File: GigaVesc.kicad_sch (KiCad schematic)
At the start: 0 parts

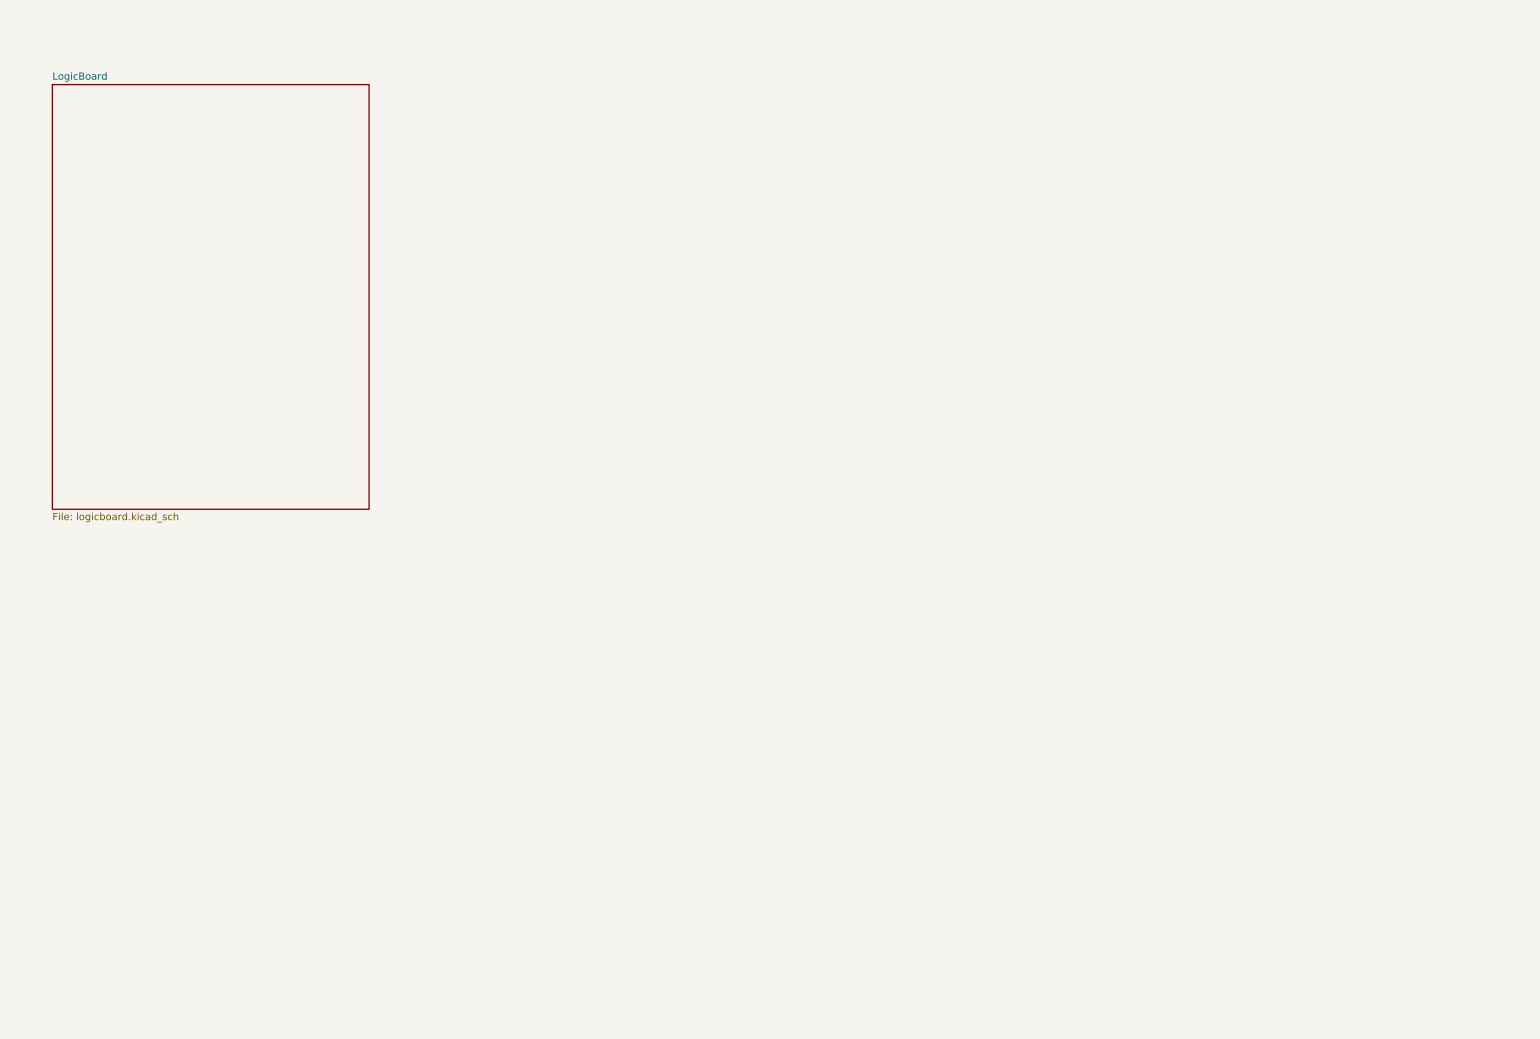
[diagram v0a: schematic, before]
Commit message: initial
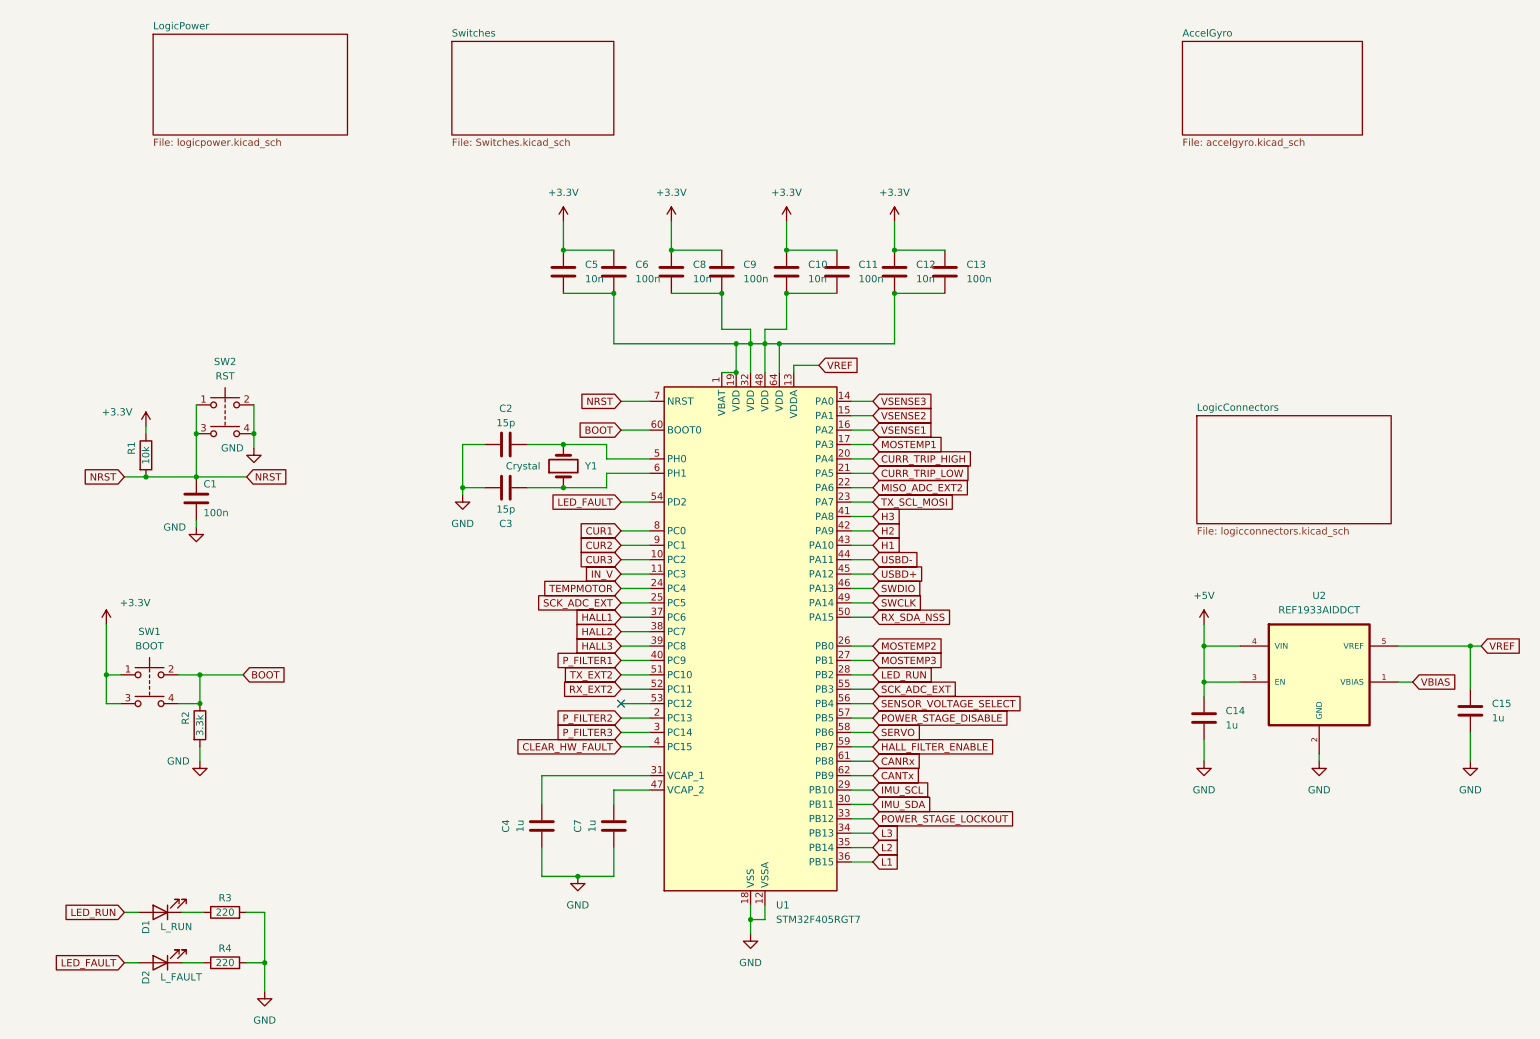
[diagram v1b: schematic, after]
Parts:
- added C1, C11, C13, C6, C9: 100n, Capacitor_SMD:C_0805_2012Metric, symbol Device:C
- added C10, C12, C5, C8: 10n, Capacitor_SMD:C_0805_2012Metric, symbol Device:C
- added C14, C15, C4, C7: 1u, Capacitor_SMD:C_0805_2012Metric, symbol Device:C
- added C2, C3: 15p, Capacitor_SMD:C_0805_2012Metric, symbol Device:C
- added D1: L_RUN, LED_SMD:LED_0805_2012Metric, symbol Device:LED
- added D2: L_FAULT, LED_SMD:LED_0805_2012Metric, symbol Device:LED
- added R1: 10k, Resistor_SMD:R_0805_2012Metric, symbol Device:R
- added R2: 3.3k, Resistor_SMD:R_0805_2012Metric, symbol Device:R
- added R3, R4: 220, Resistor_SMD:R_0805_2012Metric, symbol Device:R
- added SW1: BOOT, Button_Switch_SMD:SW_SPST_CK_RS282G05A3, symbol Switch:SW_Push_Dual
- added SW2: RST, Button_Switch_SMD:SW_SPST_CK_RS282G05A3, symbol Switch:SW_Push_Dual
- added U1: STM32F405RGT7, Package_QFP:LQFP-64_10x10mm_P0.5mm, symbol MCU_ST_STM32F4:STM32F405RGTx
- added U2: REF1933AIDDCT, Package_TO_SOT_SMD:SOT-23-5, symbol GigaVescSymbols:REF1933AIDDCT
- added Y1: Crystal, Crystal:Crystal_SMD_HC49-SD, symbol Device:Crystal
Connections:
- new net: C10.2, C11.2, C12.2, C13.2, C5.2, C6.2, C8.2, C9.2, U1.1 (VBAT), U1.19 (VDD), U1.32 (VDD), U1.48 (VDD), U1.64 (VDD)
- new net: D2.1 (K), R4.1
- new net: C2.1, U1.5 (PH0), Y1.2
- new net: D1.1 (K), R3.1
- new net: C4.1, U1.31 (VCAP_1)
- new net: C7.1, U1.47 (VCAP_2)
- new net: C3.2, U1.6 (PH1), Y1.1
- new net +3.3V: C10.1, C11.1, C12.1, C13.1, C5.1, C6.1, C8.1, C9.1, R1.1, SW1.1, SW1.3
- new net +5V: C14.1, U2.3 (EN), U2.4 (VIN)
- new net BOOT: R2.1, SW1.2, SW1.4, U1.60 (BOOT0)
- new net CANRx: U1.61 (PB8)
- new net CANTx: U1.62 (PB9)
- new net CLEAR_HW_FAULT: U1.4 (PC15)
- new net CUR1: U1.8 (PC0)
- new net CUR2: U1.9 (PC1)
- new net CUR3: U1.10 (PC2)
- new net CURR_TRIP_HIGH: U1.20 (PA4)
- new net CURR_TRIP_LOW: U1.21 (PA5)
- new net GND: C1.2, C14.2, C15.2, C2.2, C3.1, C4.2, C7.2, R2.2, R3.2, R4.2, SW2.2, SW2.4, U1.12 (VSSA), U1.18 (VSS), U1.63 (VSS), U2.2 (GND)
- new net H1: U1.43 (PA10)
- new net H2: U1.42 (PA9)
- new net H3: U1.41 (PA8)
- new net HALL1: U1.37 (PC6)
- new net HALL2: U1.38 (PC7)
- new net HALL3: U1.39 (PC8)
- new net HALL_FILTER_ENABLE: U1.59 (PB7)
- new net IMU_SCL: U1.29 (PB10)
- new net IMU_SDA: U1.30 (PB11)
- new net IN_V: U1.11 (PC3)
- new net L1: U1.36 (PB15)
- new net L2: U1.35 (PB14)
- new net L3: U1.34 (PB13)
- new net LED_FAULT: D2.2 (A), U1.54 (PD2)
- new net LED_RUN: D1.2 (A), U1.28 (PB2)
- new net MISO_ADC_EXT2: U1.22 (PA6)
- new net MOSTEMP1: U1.17 (PA3)
- new net MOSTEMP2: U1.26 (PB0)
- new net MOSTEMP3: U1.27 (PB1)
- new net NRST: C1.1, R1.2, SW2.1, SW2.3, U1.7 (NRST)
- new net POWER_STAGE_DISABLE: U1.57 (PB5)
- new net POWER_STAGE_LOCKOUT: U1.33 (PB12)
- new net P_FILTER1: U1.40 (PC9)
- new net P_FILTER2: U1.2 (PC13)
- new net P_FILTER3: U1.3 (PC14)
- new net RX_EXT2: U1.52 (PC11)
- new net RX_SDA_NSS: U1.50 (PA15)
- new net SCK_ADC_EXT: U1.25 (PC5), U1.55 (PB3)
- new net SENSOR_VOLTAGE_SELECT: U1.56 (PB4)
- new net SERVO: U1.58 (PB6)
- new net SWCLK: U1.49 (PA14)
- new net SWDIO: U1.46 (PA13)
- new net TEMPMOTOR: U1.24 (PC4)
- new net TX_EXT2: U1.51 (PC10)
- new net TX_SCL_MOSI: U1.23 (PA7)
- new net USBD+: U1.45 (PA12)
- new net USBD-: U1.44 (PA11)
- new net VBIAS: U2.1 (VBIAS)
- new net VREF: C15.1, U1.13 (VDDA), U2.5 (VREF)
- new net VSENSE1: U1.16 (PA2)
- new net VSENSE2: U1.15 (PA1)
- new net VSENSE3: U1.14 (PA0)
- no-connect marks 0 -> 1
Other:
- removed sheet LogicBoard
- added sheet AccelGyro (accelgyro.kicad_sch)
- added sheet LogicConnectors (logicconnectors.kicad_sch)
- added sheet LogicPower (logicpower.kicad_sch)
- added sheet Switches (Switches.kicad_sch)

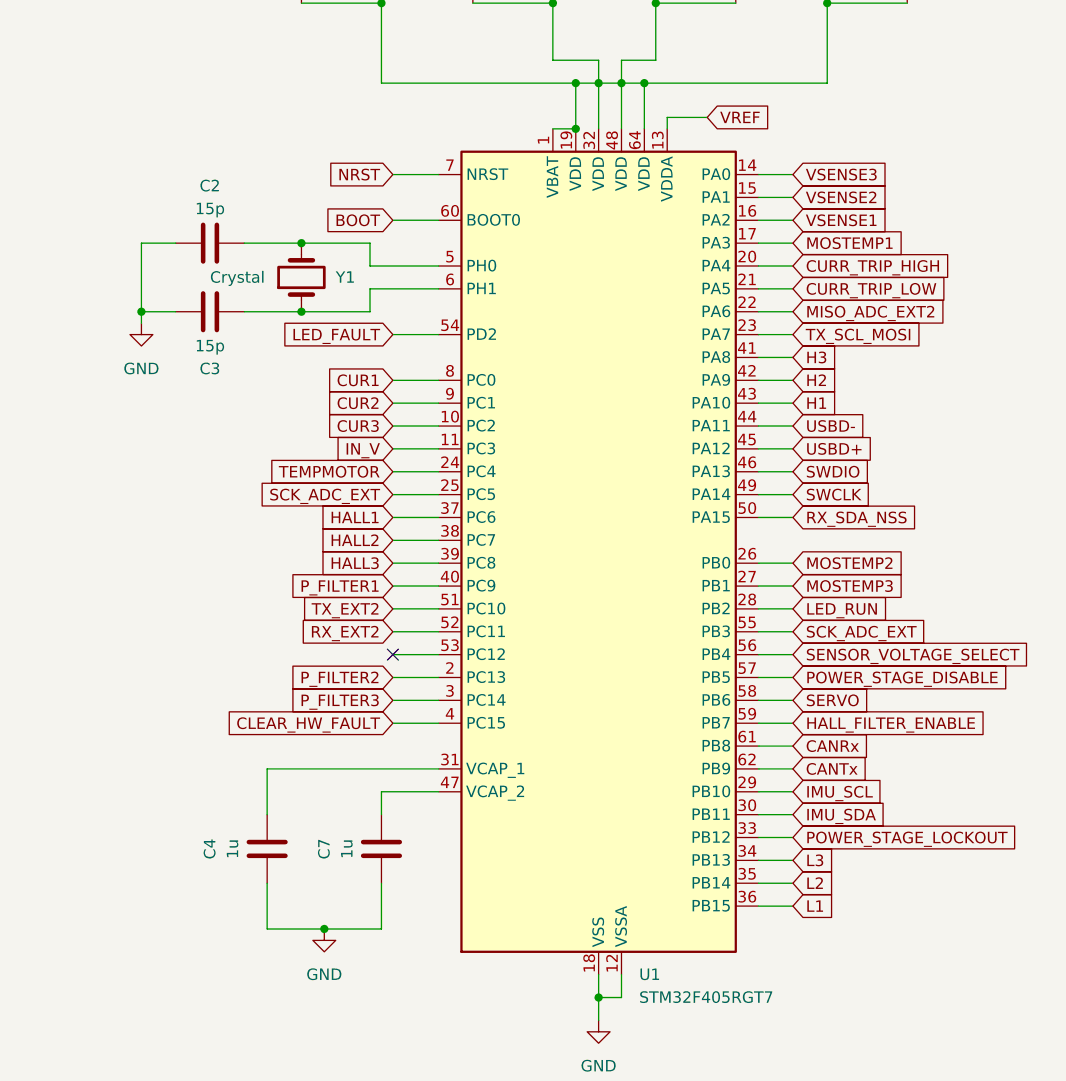
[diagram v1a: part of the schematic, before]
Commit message: initial
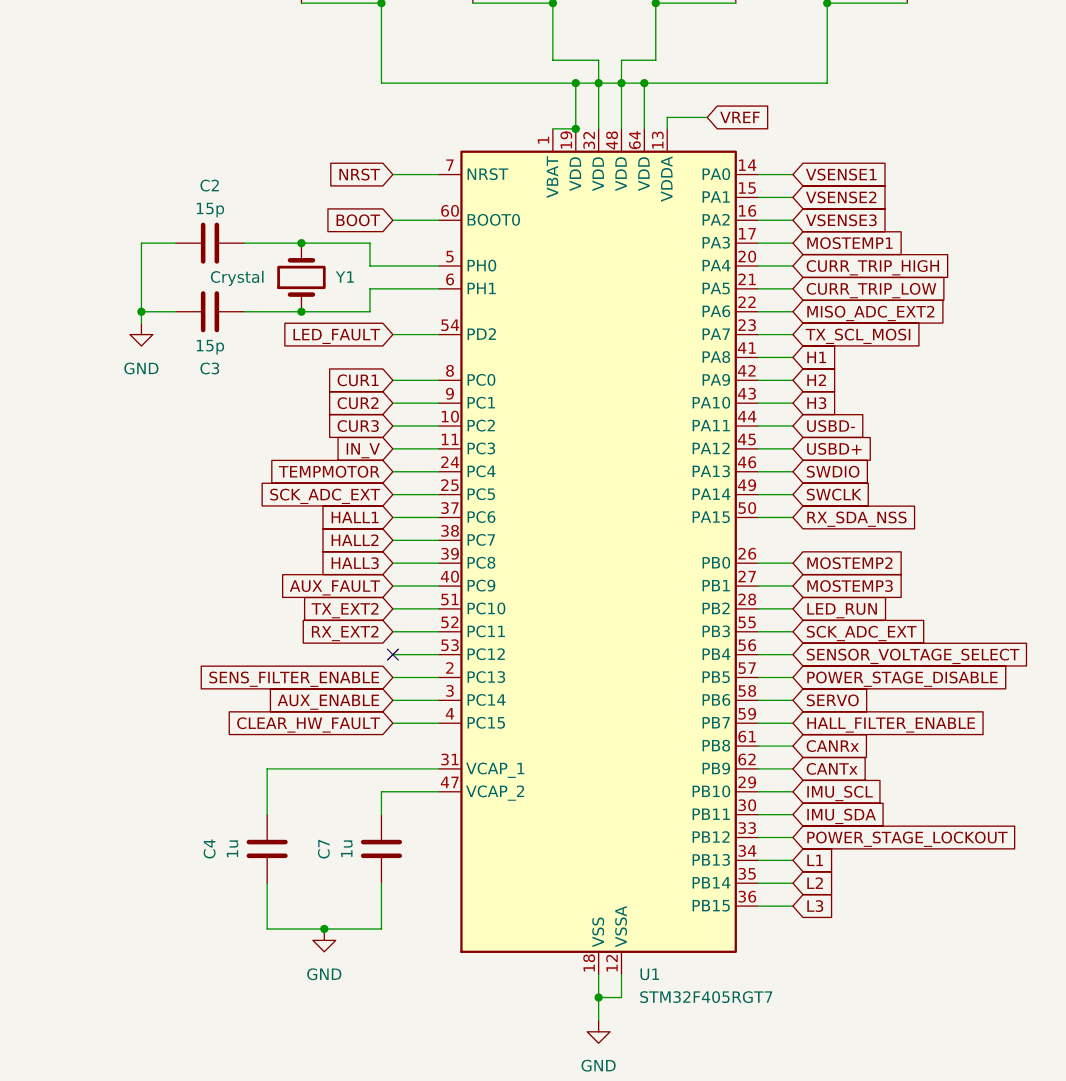
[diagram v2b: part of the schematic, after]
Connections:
- net H1: now also U1.41 (PA8); no longer U1.43 (PA10)
- net H3: now also U1.43 (PA10); no longer U1.41 (PA8)
- net L1: now also U1.34 (PB13); no longer U1.36 (PB15)
- net L3: now also U1.36 (PB15); no longer U1.34 (PB13)
- net VSENSE1: now also U1.14 (PA0); no longer U1.16 (PA2)
- net VSENSE3: now also U1.16 (PA2); no longer U1.14 (PA0)
- net P_FILTER1 renamed AUX_FAULT
- net P_FILTER2 renamed SENS_FILTER_ENABLE
- net P_FILTER3 renamed AUX_ENABLE
